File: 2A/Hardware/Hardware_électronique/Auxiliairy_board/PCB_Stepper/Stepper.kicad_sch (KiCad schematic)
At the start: 45 parts, among them J1 UART_IN, J2 Conn_ST_STDC14, J3 Conn_01x03_Pin, J4 Conn_01x03_Pin, U4 AZ1117-3.3, U5 STM32G071CBUx

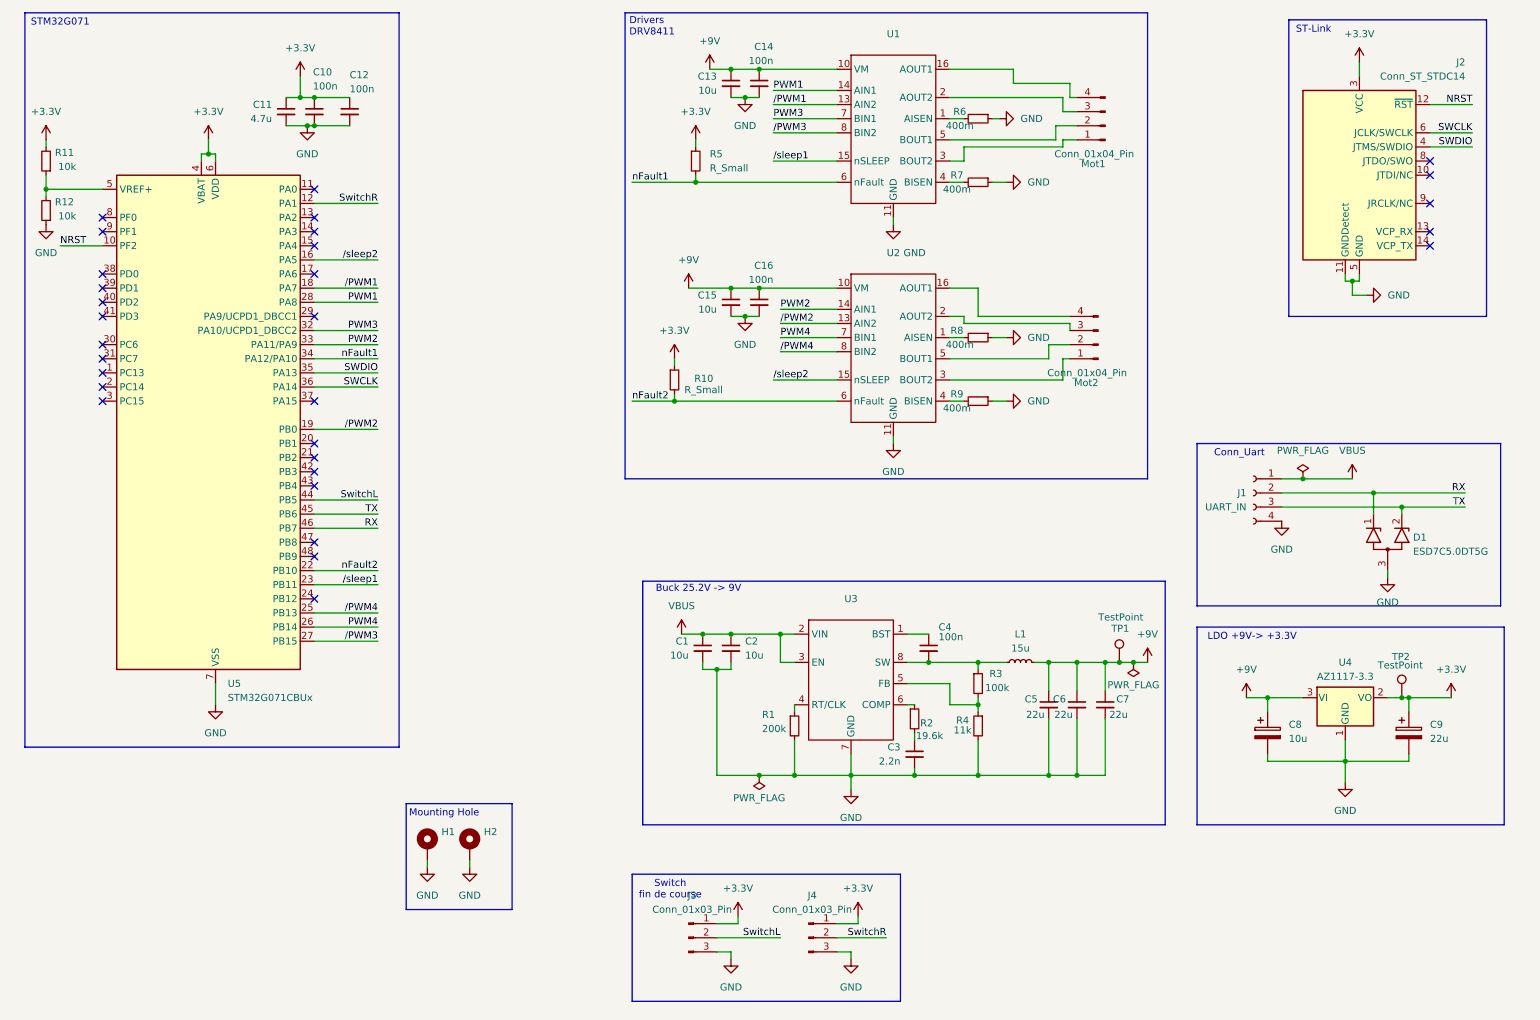
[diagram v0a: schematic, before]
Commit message: recommit to be sure...
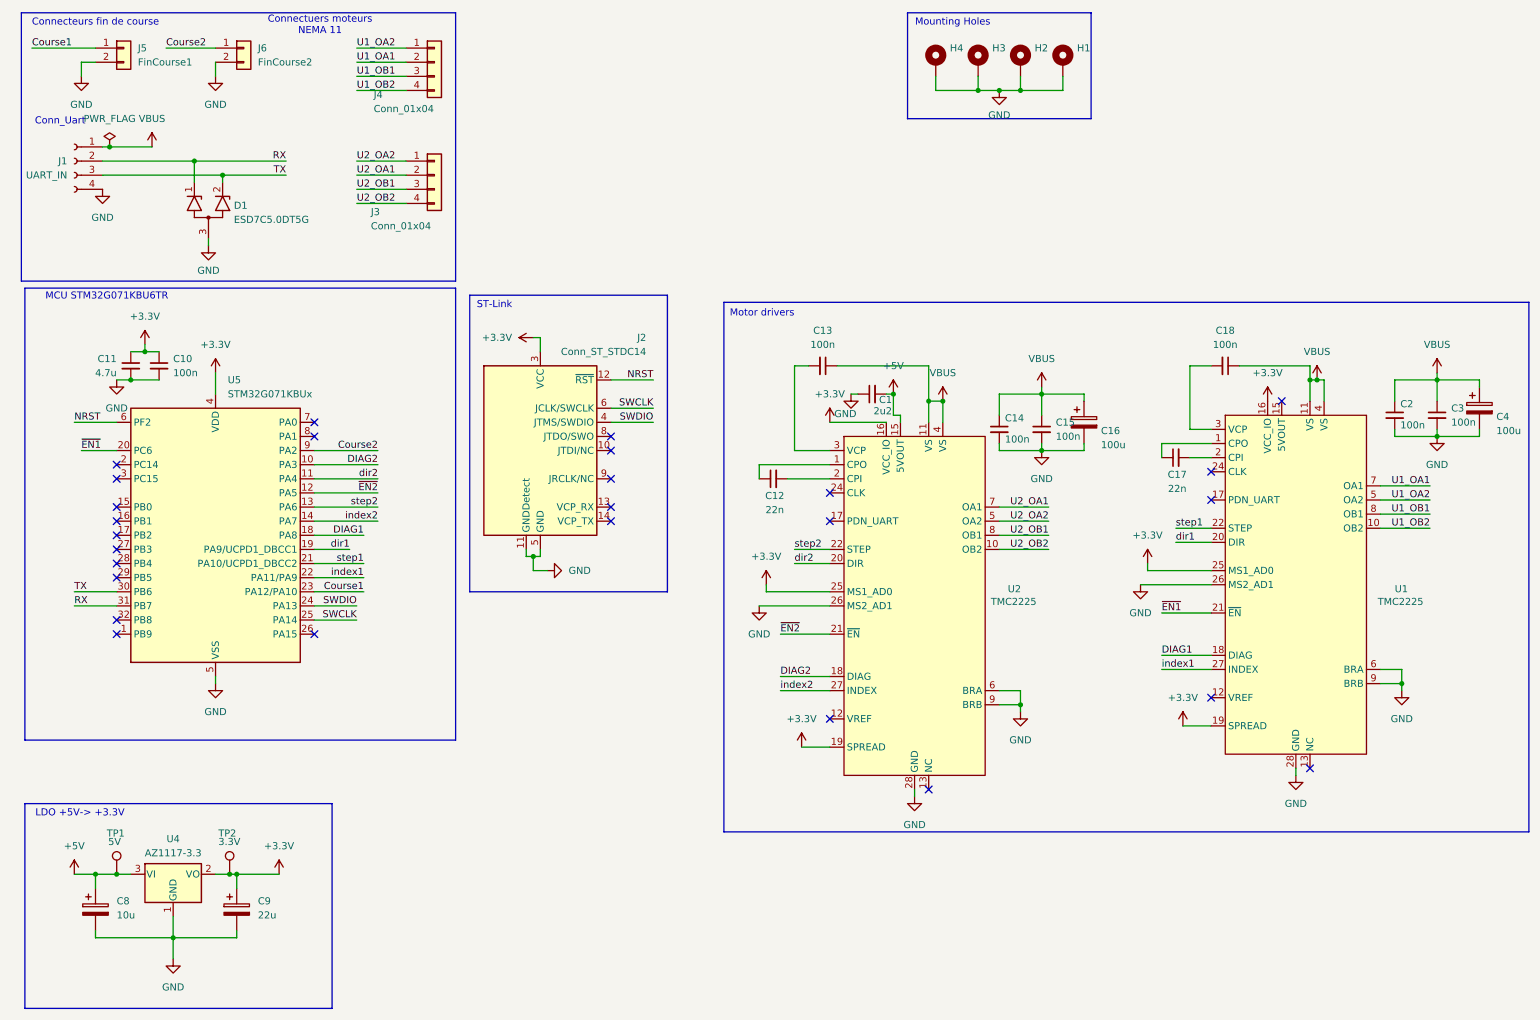
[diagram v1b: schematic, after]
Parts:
- removed C16, C4: 100n, Capacitor_SMD:C_0402_1005Metric, symbol Device:C_Small
- removed C5, C6, C7: 22u, Capacitor_SMD:C_0805_2012Metric, symbol Device:C_Small
- removed J3, J4: Conn_01x03_Pin, Connector_JST:JST_EH_B3B-EH-A_1x03_P2.50mm_Vertical, symbol Connector:Conn_01x03_Pin
- removed L1: 15u, MainBoard:PA5432.472NLT, symbol Device:L_Small
- removed Mot1, Mot2: Conn_01x04_Pin, Connector_JST:JST_EH_B4B-EH-A_1x04_P2.50mm_Vertical, symbol Connector:Conn_01x04_Pin
- removed R1: 200k, Resistor_SMD:R_0402_1005Metric, symbol Device:R_Small
- removed R10, R5: R_Small, Resistor_SMD:R_0402_1005Metric, symbol Device:R_Small
- removed R11, R12: 10k, Resistor_SMD:R_0402_1005Metric, symbol Device:R_Small
- removed R2: 19.6k, Resistor_SMD:R_0402_1005Metric, symbol Device:R_Small
- removed R3: 100k, Resistor_SMD:R_0402_1005Metric, symbol Device:R_Small
- removed R4: 11k, Resistor_SMD:R_0402_1005Metric, symbol Device:R_Small
- removed R6, R7, R8, R9: 400m, Resistor_SMD:R_0402_1005Metric, symbol Device:R_Small
- removed U1, U2: ~, Package_DFN_QFN:WQFN-16-1EP_3x3mm_P0.5mm_EP1.68x1.68mm, symbol Stepper:DRV8411
- removed U3: ~, Package_SO:SOIC-8-1EP_3.9x4.9mm_P1.27mm_EP2.95x4.9mm_Mask2.71x3.4mm, symbol Custom:AP64500Q
- removed U5: STM32G071CBUx, Package_DFN_QFN:QFN-48-1EP_7x7mm_P0.5mm_EP5.6x5.6mm, symbol MCU_ST_STM32G0:STM32G071CBUx
- added C16, C4: 100u, Capacitor_SMD:CP_Elec_10x10.5, symbol Device:C_Polarized
- added C17: 22n, Capacitor_SMD:C_0603_1608Metric_Pad1.08x0.95mm_HandSolder, symbol Device:C_Small
- added C18: 100n, Capacitor_SMD:C_0603_1608Metric_Pad1.08x0.95mm_HandSolder, symbol Device:C_Small
- added H3, H4: MountingHole_Pad, MountingHole:MountingHole_2.7mm_M2.5_ISO7380_Pad, symbol Mechanical:MountingHole_Pad
- added J3, J4: Conn_01x04, Connector_JST:JST_EH_B4B-EH-A_1x04_P2.50mm_Vertical, symbol Connector_Generic:Conn_01x04
- added J5: FinCourse1, Connector_JST:JST_EH_B2B-EH-A_1x02_P2.50mm_Vertical, symbol Connector_Generic:Conn_01x02
- added J6: FinCourse2, Connector_JST:JST_EH_B2B-EH-A_1x02_P2.50mm_Vertical, symbol Connector_Generic:Conn_01x02
- added U1, U2: TMC2225, Package_SO:HTSSOP-28-1EP_4.4x9.7mm_P0.65mm_EP2.75x6.2mm_ThermalVias, symbol Custom:TMC2225
- added U5: STM32G071KBUx, Package_DFN_QFN:QFN-32-1EP_5x5mm_P0.5mm_EP3.45x3.45mm, symbol MCU_ST_STM32G0:STM32G071KBUx
- C1: value 10u -> 2u2; footprint Capacitor_SMD:C_0805_2012Metric -> Capacitor_SMD:C_0402_1005Metric
- C11: footprint Resistor_SMD:R_0402_1005Metric -> Capacitor_SMD:C_0402_1005Metric
- C12: value 100n -> 22n; footprint Capacitor_SMD:C_0402_1005Metric -> Capacitor_SMD:C_0603_1608Metric
- C13, C15, C2: value 10u -> 100n; footprint Capacitor_SMD:C_0805_2012Metric -> Capacitor_SMD:C_0603_1608Metric
- C14: footprint Capacitor_SMD:C_0402_1005Metric -> Capacitor_SMD:C_0603_1608Metric
- C3: value 2.2n -> 100n; footprint Capacitor_SMD:C_0402_1005Metric -> Capacitor_SMD:C_0603_1608Metric
- C8: footprint Capacitor_SMD:C_0805_2012Metric -> Capacitor_SMD:C_0805_2012Metric_Pad1.18x1.45mm_HandSolder
- H1, H2: footprint MountingHole:MountingHole_2.7mm_M2.5_Pad -> MountingHole:MountingHole_2.7mm_M2.5_ISO7380_Pad
- TP1: value TestPoint -> 5V
- TP2: value TestPoint -> 3.3V
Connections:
- net +3.3V: now also U1.16 (VCC_IO), U1.19 (SPREAD), U1.25 (MS1_AD0), U2.16 (VCC_IO), U2.19 (SPREAD), U2.25 (MS1_AD0), U5.4 (VDD); no longer C12.1
- net GND: now also C1.1, C16.2, C4.2, H3.1, H4.1, J5.2 (Pin_2), J6.2 (Pin_2), U1.14 (GND), U1.26 (MS2_AD1), U1.28 (GND), U1.29 (GND), U1.6 (BRA), U1.9 (BRB), U2.14 (GND), U2.26 (MS2_AD1), U2.28 (GND), U2.29 (GND), U2.6 (BRA), U2.9 (BRB), U5.33 (VSS), U5.5 (VSS); no longer C1.2, C12.2, C13.2
- net NRST: now also U5.6 (PF2)
- net RX: now also U5.31 (PB7)
- net SWCLK: now also U5.25 (PA14)
- net SWDIO: now also U5.24 (PA13)
- net TX: now also U5.30 (PB6)
- net VBUS: now also C13.1, C14.1, C15.1, C3.1, C16.1, C18.1, C4.1, U1.11 (VS), U1.4 (VS), U2.11 (VS), U2.4 (VS); no longer C1.1
- net +9V renamed +5V
- net +5V: now also C1.2, U2.15 (5VOUT); no longer C13.1, C14.1, C15.1
- new net: C17.1, U1.1 (CPO)
- new net: C17.2, U1.2 (CPI)
- new net: C12.1, U2.1 (CPO)
- new net: C12.2, U2.2 (CPI)
- new net: C13.2, U2.3 (VCP)
- new net: C18.2, U1.3 (VCP)
- new net Course1: J5.1 (Pin_1), U5.23 (PA12/PA10)
- new net Course2: J6.1 (Pin_1), U5.9 (PA2)
- new net DIAG1: U1.18 (DIAG), U5.18 (PA8)
- new net DIAG2: U2.18 (DIAG), U5.10 (PA3)
- new net U1_OA1: J4.2 (Pin_2), U1.7 (OA1)
- new net U1_OA2: J4.1 (Pin_1), U1.5 (OA2)
- new net U1_OB1: J4.3 (Pin_3), U1.8 (OB1)
- new net U1_OB2: J4.4 (Pin_4), U1.10 (OB2)
- new net U2_OA1: J3.2 (Pin_2), U2.7 (OA1)
- new net U2_OA2: J3.1 (Pin_1), U2.5 (OA2)
- new net U2_OB1: J3.3 (Pin_3), U2.8 (OB1)
- new net U2_OB2: J3.4 (Pin_4), U2.10 (OB2)
- new net dir1: U1.20 (DIR), U5.19 (PA9/UCPD1_DBCC1)
- new net dir2: U2.20 (DIR), U5.11 (PA4)
- new net index1: U1.27 (INDEX), U5.22 (PA11/PA9)
- new net index2: U2.27 (INDEX), U5.14 (PA7)
- new net step1: U1.22 (STEP), U5.21 (PA10/UCPD1_DBCC2)
- new net step2: U2.22 (STEP), U5.13 (PA6)
- new net ~{EN1}: U1.21 (~{EN}), U5.20 (PC6)
- new net ~{EN2}: U2.21 (~{EN}), U5.12 (PA5)
- no-connect marks 30 -> 27
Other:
- note added: "Connecteurs fin de course"
- note added: "Connectuers moteurs NEMA 11"
- note added: "LDO +5V-> +3.3V"
- note added: "MCU STM32G071KBU6TR"
- note added: "Motor drivers"
- note added: "Mounting Holes"
- note removed: "Buck 25.2V -> 9V"
- note removed: "Drivers DRV8411"
- note removed: "LDO +9V-> +3.3V"
- note removed: "Mounting Hole"
- note removed: "STM32G071"
- note removed: "Switch fin de course"
- moved on the sheet: C10, C11, C8, C9, D1, J1, J2, TP2, U4
